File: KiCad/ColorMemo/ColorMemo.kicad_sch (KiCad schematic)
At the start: 49 parts, among them SW1 SW_Push, SW10 SW_Push, SW11 SW_Push, SW12 SW_Push, SW13 SW_Push, SW14 SW_Push, SW15 SW_Push, SW16 SW_Push, SW17 SW_Push, SW18 SW_Push, SW19 SW_Push, SW2 SW_Push, SW20 SW_Push, SW21 SW_Push, SW22 SW_Push, SW23 SW_Push, SW24 SW_Push, SW3 SW_Push, SW4 SW_Push, SW5 SW_Push, SW6 SW_Push, SW7 SW_Push, SW8 SW_Push, SW9 SW_Push, U1 WEMOS_D1_mini

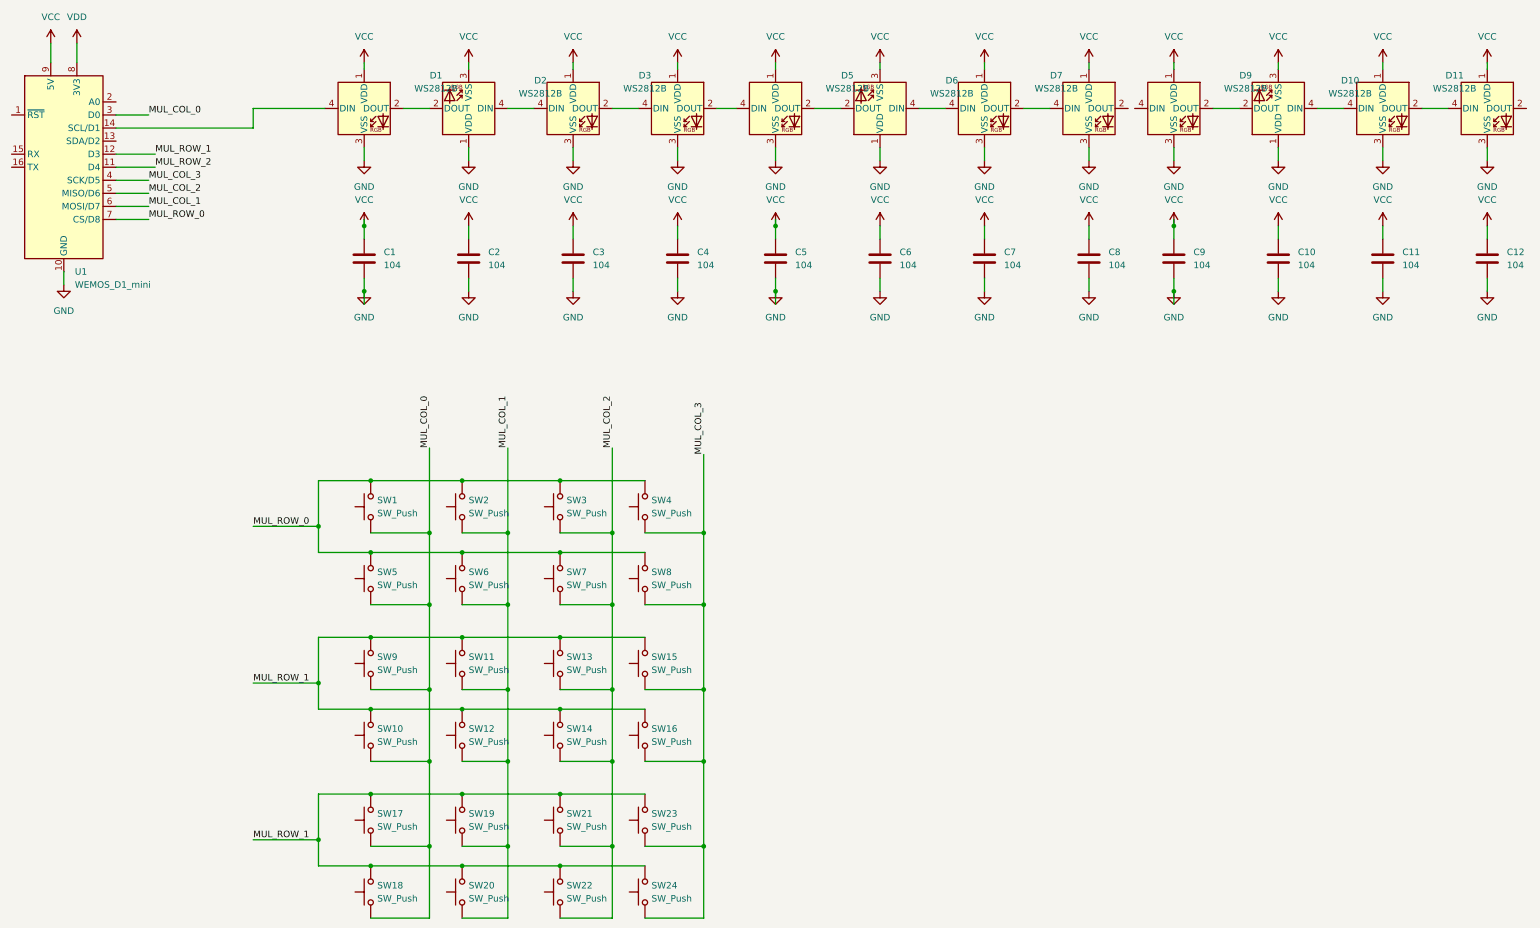
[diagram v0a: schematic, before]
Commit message: added kicad project
Signed-off-by: Michal Pelka <michalpelka@gmail.com>
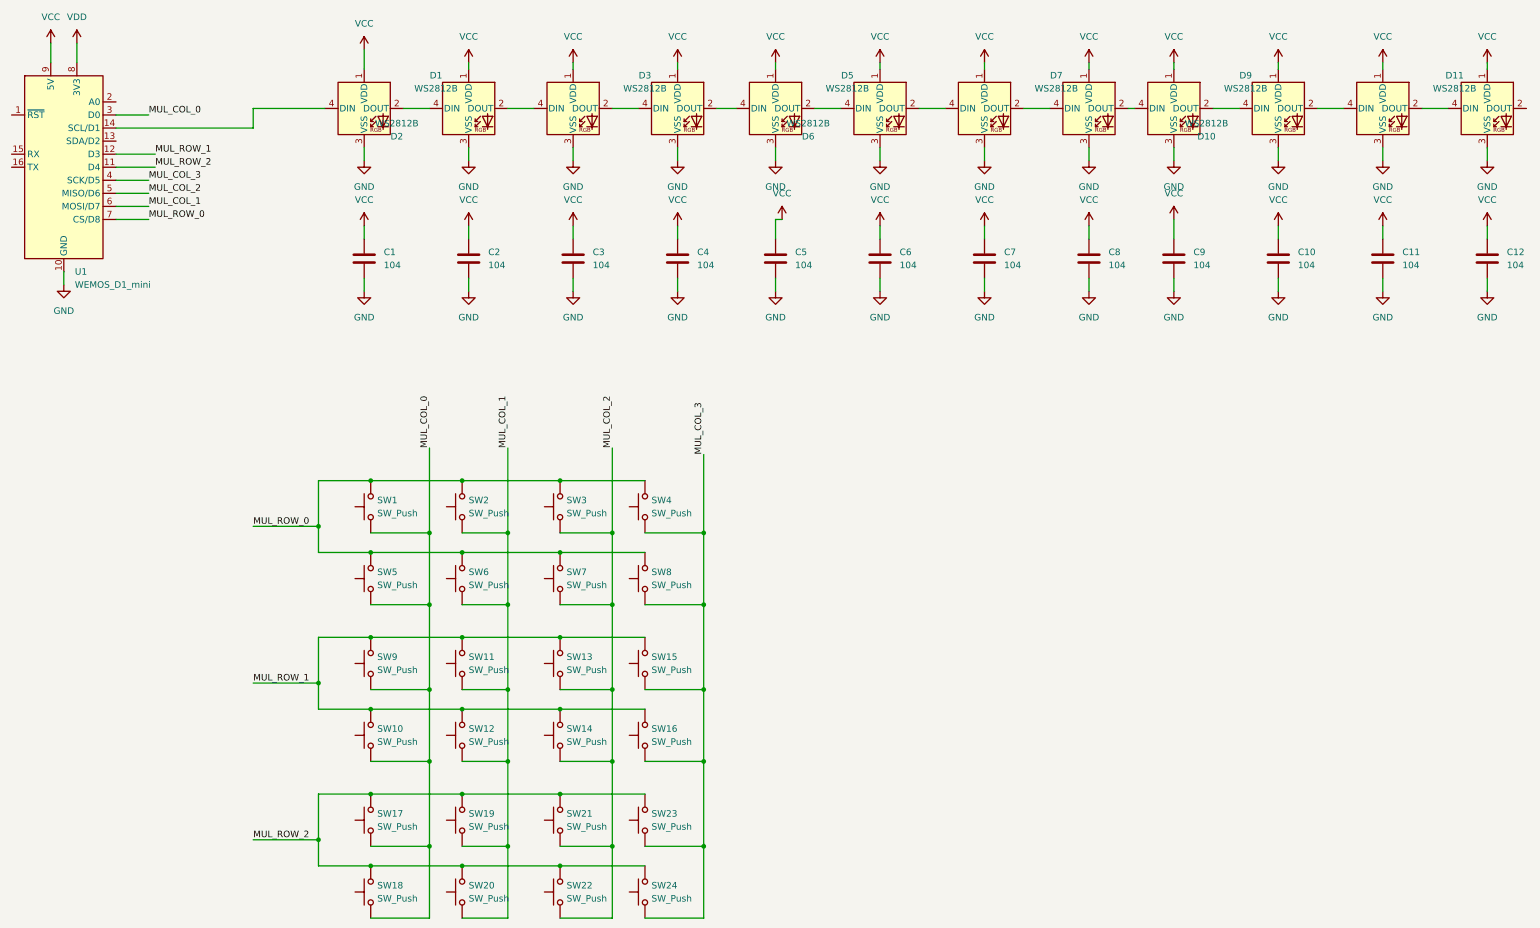
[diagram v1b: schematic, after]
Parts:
- SW1, SW10, SW11, SW12, SW13, SW14, SW15, SW16, SW17, SW18, SW19, SW2, SW20, SW21, SW22, SW23, SW24, SW3, SW4, SW5, SW6, SW7, SW8, SW9: footprint Button_Switch_THT:SW_PUSH-12mm -> Button_Switch_THT:SW_PUSH_6mm
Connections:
- net GND: now also D10.3 (VSS), D2.3 (VSS), D6.3 (VSS); no longer D10.1 (VDD), D2.1 (VDD), D6.1 (VDD)
- net MUL_ROW_1: no longer SW17.2, SW18.2, SW19.2, SW20.2, SW21.2, SW22.2, SW23.2, SW24.2
- net MUL_ROW_2: now also SW17.2, SW18.2, SW19.2, SW20.2, SW21.2, SW22.2, SW23.2, SW24.2
- net VCC: now also D10.1 (VDD), D2.1 (VDD), D6.1 (VDD); no longer D10.3 (VSS), D2.3 (VSS), D6.3 (VSS)
- net at D3.4 (DIN): now also D2.2 (DOUT); no longer D2.4 (DIN)
- net at D10.2 (DOUT): now also D11.4 (DIN); no longer D9.2 (DOUT)
- net at D10.4 (DIN): now also D9.2 (DOUT); no longer D11.4 (DIN)
- net at D6.2 (DOUT): now also D7.4 (DIN); no longer D5.2 (DOUT)
- net at D6.4 (DIN): now also D5.2 (DOUT); no longer D7.4 (DIN)
- net at D1.2 (DOUT): now also D2.4 (DIN); no longer D2.2 (DOUT)
- net at D8.2 (DOUT): now also D9.4 (DIN)
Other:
- moved on the sheet: D10, D2, D6
